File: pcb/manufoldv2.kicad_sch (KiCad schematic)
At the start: 3 parts, among them U1 ProMicro

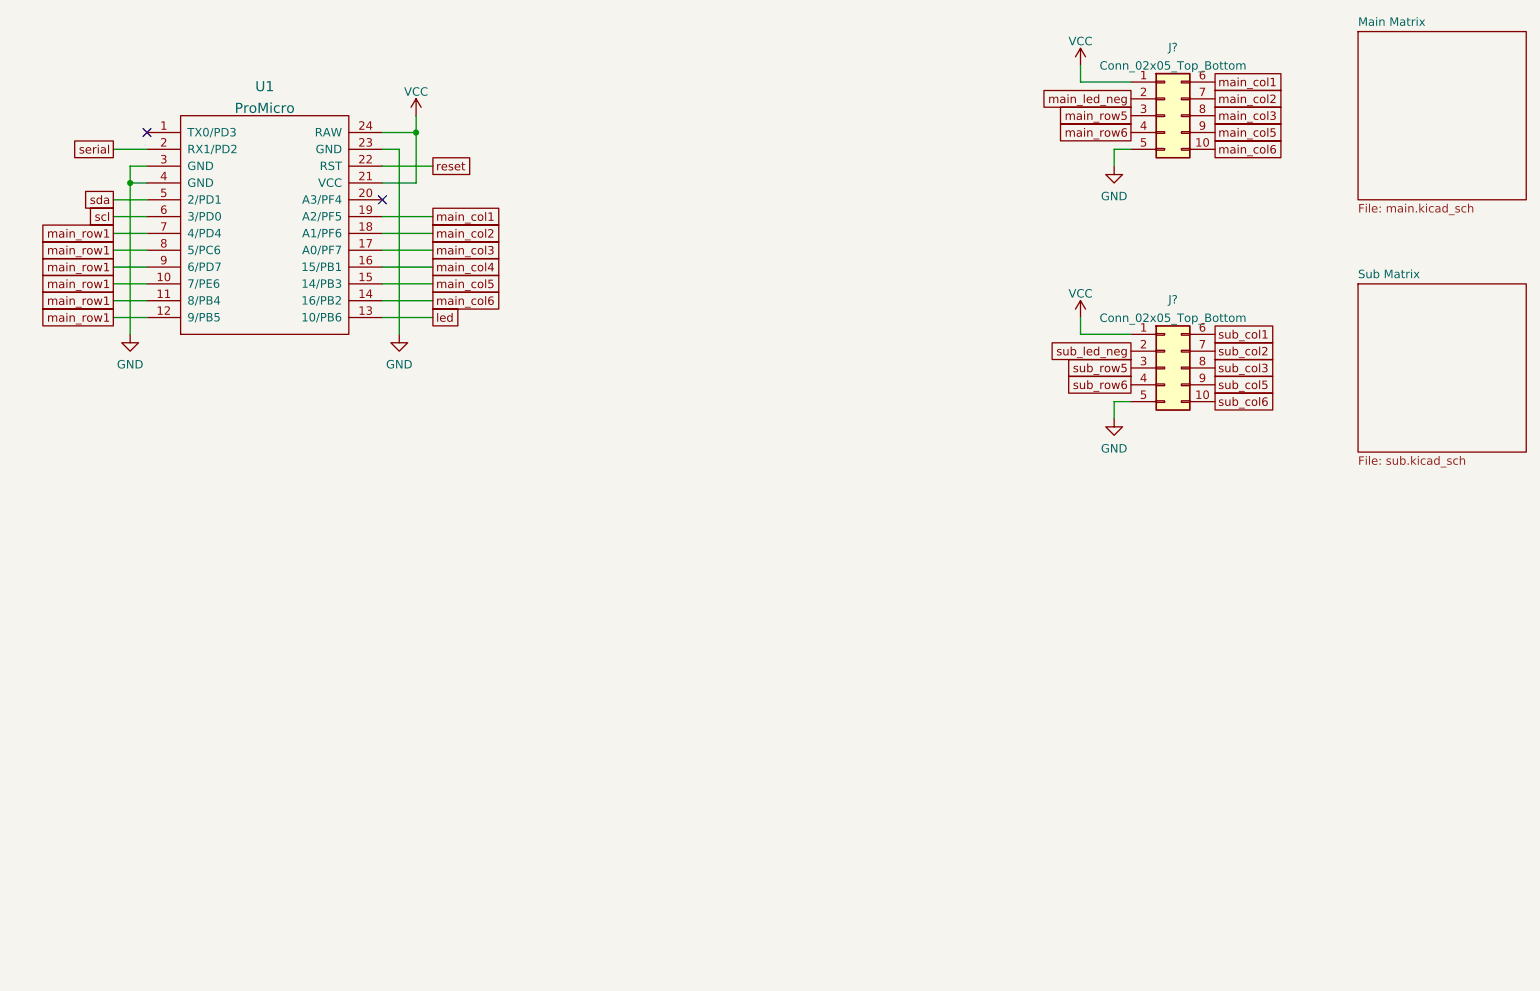
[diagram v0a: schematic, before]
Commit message: initial schematic
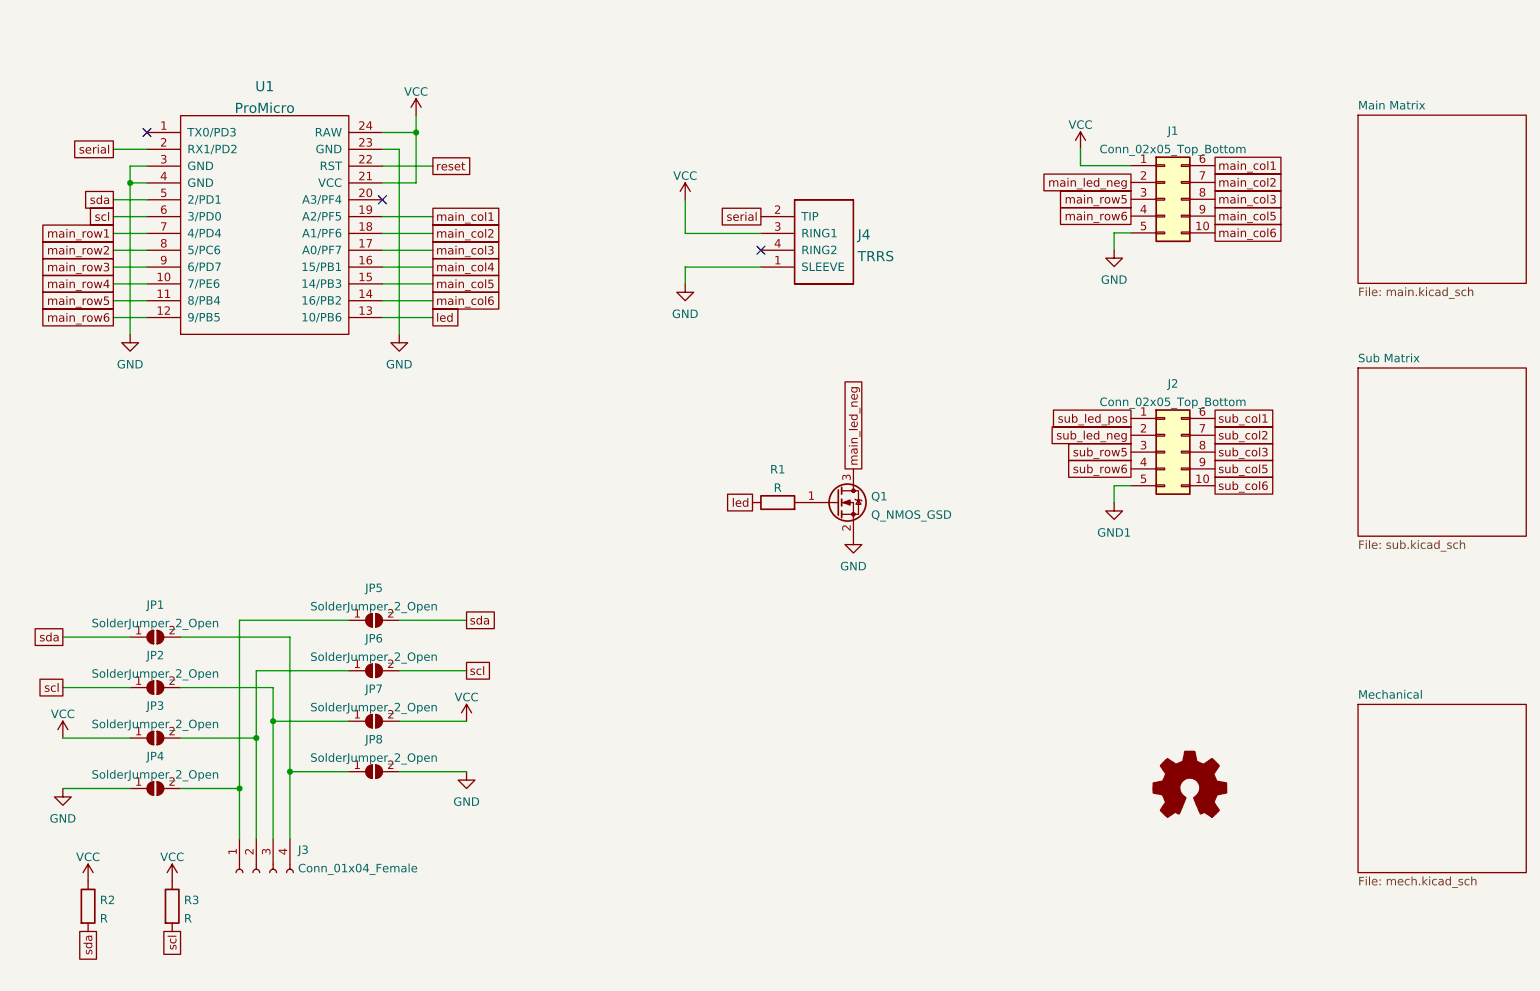
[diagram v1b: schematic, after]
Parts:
- added J3: Conn_01x04_Female, symbol Connector:Conn_01x04_Female
- added J4: TRRS, symbol keebio:TRRS
- added JP1, JP2, JP3, JP4, JP5, JP6, JP7, JP8: SolderJumper_2_Open, symbol Jumper:SolderJumper_2_Open
- added Q1: Q_NMOS_GSD, symbol Device:Q_NMOS_GSD
- added R1, R2, R3: R, symbol Device:R
- gave numbers to parts that had none: 2
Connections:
- net GND: now also J4.1 (SLEEVE), JP4.1 (A), JP8.2 (B), Q1.2 (S); no longer J2.5 (Pin_5)
- net VCC: now also J4.3 (RING1), JP3.1 (A), JP7.2 (B), R2.1, R3.1; no longer J2.1 (Pin_1)
- net led: now also R1.1
- net main_led_neg: now also Q1.3 (D)
- net main_row1: no longer U1.10 (7/PE6), U1.11 (8/PB4), U1.12 (9/PB5), U1.8 (5/PC6), U1.9 (6/PD7)
- net main_row5: now also U1.11 (8/PB4)
- net main_row6: now also U1.12 (9/PB5)
- net scl: now also JP2.1 (A), JP6.2 (B), R3.2
- net sda: now also JP1.1 (A), JP5.2 (B), R2.2
- net serial: now also J4.2 (TIP)
- new net: J3.1 (Pin_1), JP4.2 (B), JP5.1 (A)
- new net: J3.2 (Pin_2), JP3.2 (B), JP6.1 (A)
- new net: J3.3 (Pin_3), JP2.2 (B), JP7.1 (A)
- new net: J3.4 (Pin_4), JP1.2 (B), JP8.1 (A)
- new net: Q1.1 (G), R1.2
- new net GND1: J2.5 (Pin_5)
- new net main_row2: U1.8 (5/PC6)
- new net main_row3: U1.9 (6/PD7)
- new net main_row4: U1.10 (7/PE6)
- new net sub_led_pos: J2.1 (Pin_1)
- no-connect marks 2 -> 3
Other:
- added sheet Mechanical (mech.kicad_sch)
- moved on the sheet: J1, J2
